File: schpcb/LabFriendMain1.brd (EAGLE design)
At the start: 100 x 100.1 mm, 654 parts, among them IC1 TPS62240DDC, IC10 TPS62240DDC, IC11 TPS73001DBVR, IC12 TPS73001DBVR, IC13 AK4621, IC14 TPS72301, IC15 LME49721, IC16 NE5532, IC17 OPA2134, IC18 LM8272, IC19 LMV358MM, IC2 25px80, IC20 ISL54405IRTZ, IC21 NE5532, IC22 74HC4052D, IC23 LME49721, IC24 74HC00D, IC25 INA331IDGK, IC26 MT41J128M8, IC27 74HCT132D, IC28 TPS72301, IC29 TPS73001DBVR, IC3 SI8462, IC30 LM8272, IC31 LMV358MM, IC32 ADS1118IDGSR, IC33 ADA4853-3RU, IC34 4052D, IC35 4052D, IC36 OPA2354, IC37 74HC595D, IC38 ADA4853-3RU, IC39 4052D, IC4 FT232H, IC40 4052D, IC41 OPA2354, IC42 74HC595D, IC43 LM321MF, IC44 74HC595D, IC5 ADC08200, IC6 ADC08200, IC7 TPS73001DBVR, IC8 93LC56SM, IC9 74LVC8T245, K1 G6K-2F-Y, K2 G6K-2F-Y, K3 G6K-2F-Y, K4 G6K-2F-Y, Q1 12MHz, Q2 FDN335N, Q3 FDN335N, T1 EFD15DCDCPM5P33EFD15, T10 BC850, T11 BC850, T12 BC856ASMD, T13 BC856ASMD, T14 BC850, T15 BC856ASMD, T16 BC850, T17 BC856ASMD, T2 BC850, T3 BC850, T4 BC850, T5 BC856ASMD, T6 BC856ASMD, T7 BC856ASMD, T8 BC850, T9 BC856ASMD, U2 6SLX9FTG256, X1 MINI-USB-32005-201, X2 31-5431-10RFX, X3 31-5431-10RFX

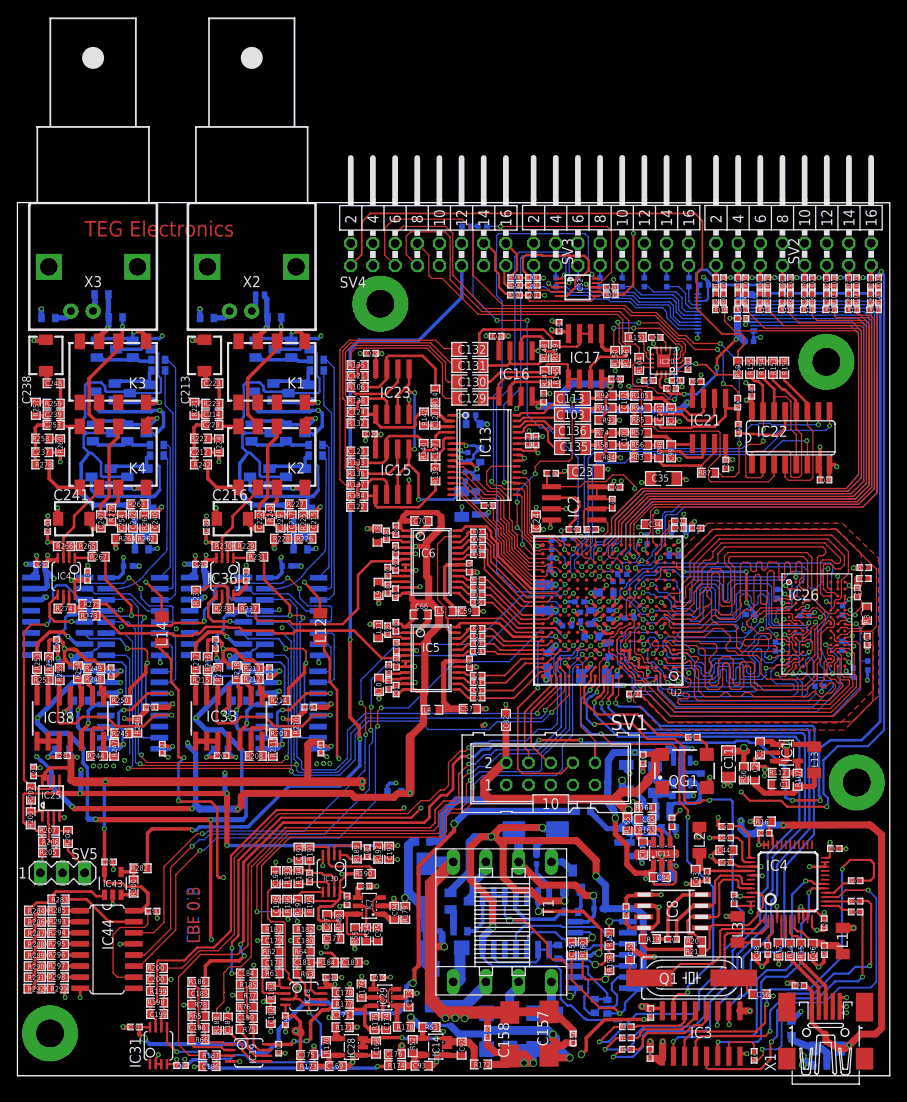
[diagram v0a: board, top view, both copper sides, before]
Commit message: Final oreder prototype
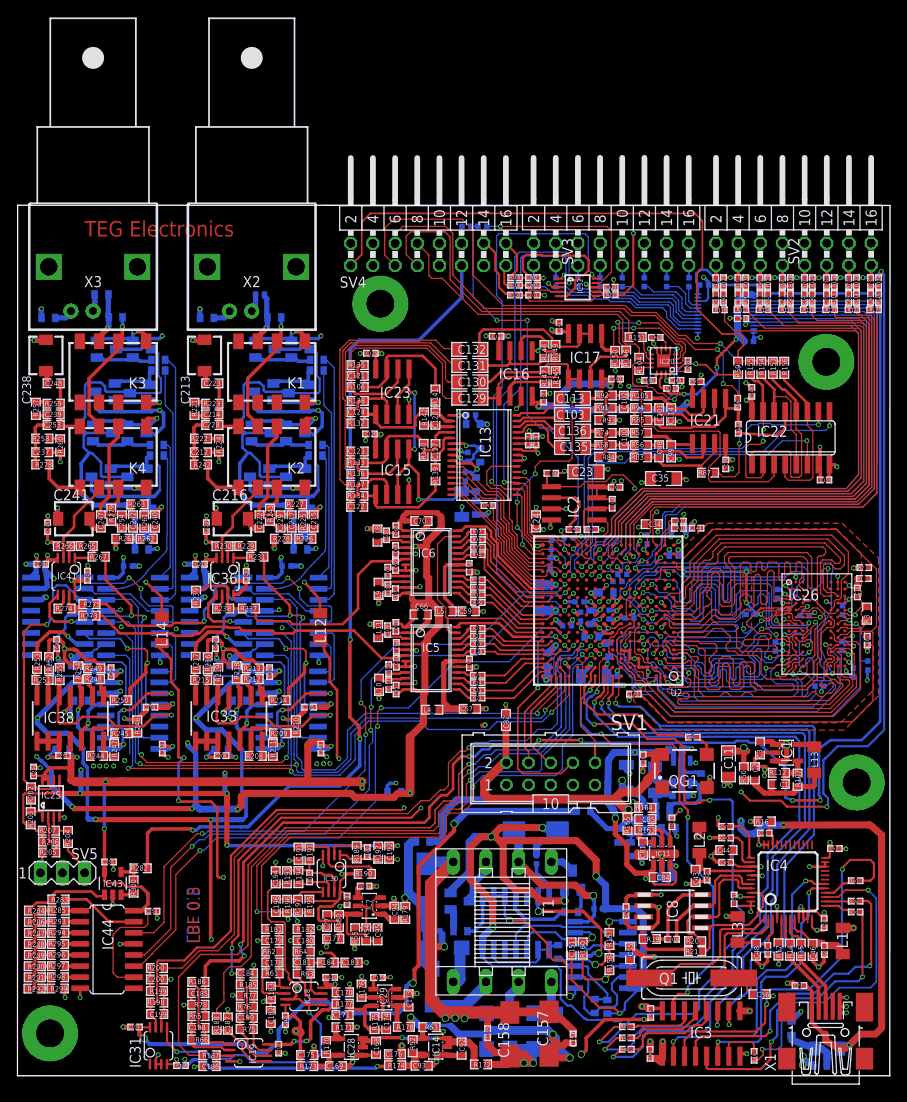
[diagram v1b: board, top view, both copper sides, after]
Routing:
- net VREFDDR: track 101.4 -> 100.4 mm
- added copper zone on layer 16, net VREFDDR
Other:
- board size 100 x 100.1 mm -> 100 x 99.8 mm
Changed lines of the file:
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@@
 <plain>
 <wire x1="60.2234" y1="0" x2="160.2032" y2="0" width="0" layer="20"/>
-<wire x1="160.2032" y1="0" x2="160.2032" y2="100.0508" width="0" layer="20"/>
-<wire x1="160.2032" y1="100.0508" x2="60.2234" y2="100.0762" width="0" layer="20"/>
-<wire x1="60.2234" y1="100.0762" x2="60.2234" y2="0" width="0" layer="20"/>
+<wire x1="160.2032" y1="0" x2="160.2282" y2="99.7508" width="0" layer="20"/>
+<wire x1="160.2282" y1="99.7508" x2="60.2484" y2="99.7762" width="0" layer="20"/>
+<wire x1="60.2484" y1="99.7762" x2="60.2234" y2="0" width="0" layer="20"/>
 <wire x1="119.0244" y1="58.0644" x2="119.0244" y2="57.8866" width="0" layer="47"/>
 <wire x1="83.6168" y1="22.1488" x2="83.4136" y2="22.1488" width="0" layer="47"/>
@@
 <vertex x="128.525" y="43.2"/>
 <vertex x="127.875" y="43.85"/>
-<vertex x="127.875" y="45.9875"/>
-<vertex x="128.2625" y="46.375"/>
-<vertex x="128.875" y="46.375"/>
-<vertex x="129.5125" y="47.0125"/>
-<vertex x="129.5125" y="49.8125"/>
-<vertex x="128.9375" y="49.975"/>
+<vertex x="127.9" y="45.7875"/>
+<vertex x="128.2375" y="46.175"/>
+<vertex x="129.175" y="46.175"/>
+<vertex x="129.175" y="46.525"/>
+<vertex x="129.0375" y="46.6625"/>
+<vertex x="128.5875" y="46.975"/>
+<vertex x="128.5375" y="49.775"/>
+<vertex x="128.375" y="49.9375"/>
 <vertex x="127.925" y="50"/>
 <vertex x="127.4875" y="50.3625"/>
@@
 <vertex x="129.725" y="55.0125"/>
 <vertex x="130.0125" y="54.575"/>
+<vertex x="129.95" y="51.2375"/>
+<vertex x="129.0125" y="50.225"/>
+<vertex x="129.0125" y="47.3125"/>
+<vertex x="129.975" y="46.35"/>
 <vertex x="129.975" y="45.7375"/>
 <vertex x="130.3625" y="45.35"/>
@@
 <via x="152.6865" y="18.7085" extent="1-16" drill="0.3048"/>
 <via x="151.003" y="23.9522" extent="1-16" drill="0.3048"/>
-<polygon width="0.254" layer="2" isolate="0.254">
+<polygon width="0.254" layer="2" isolate="0.15">
 <vertex x="137.2362" y="29.8704"/>
 <vertex x="136.9544" y="29.2612"/>
@@
 <via x="141.4526" y="18.288" extent="1-16" drill="0.3048"/>
 <via x="133.7726" y="19.3301" extent="1-16" drill="0.3048"/>
-<polygon width="0.2032" layer="3" isolate="0.254">
+<polygon width="0.2032" layer="3" isolate="0.15">
 <vertex x="152.2984" y="29.845"/>
 <vertex x="148.6662" y="29.8704"/>
@@
 <wire x1="156.45" y1="56.9999" x2="156.727" y2="57.0125" width="0.6096" layer="1"/>
 <contactref element="R50" pad="2"/>
-<polygon width="0.4064" layer="3" isolate="0.254">
-<vertex x="132.9625" y="42.6"/>
+<polygon width="0.4064" layer="3" isolate="0.15">
+<vertex x="132.4875" y="44.2625"/>
+<vertex x="131.8375" y="44.3"/>
+<vertex x="131.575" y="44.5625"/>
+<vertex x="129.425" y="44.5625"/>
+<vertex x="132.9375" y="41.05"/>
 <vertex x="132.9375" y="41"/>
 <vertex x="134.15" y="39.6125"/>
@@
 <vertex x="132.8375" y="49.8875"/>
 <vertex x="133.025" y="46.9375"/>
-<vertex x="132.95" y="43.625"/>
+<vertex x="133.05" y="44.675"/>
 </polygon>
 <wire x1="143.475" y1="35.4499" x2="143.475" y2="37.2125" width="0.6096" layer="1"/>
@@
 <wire x1="155.6625" y1="50.9375" x2="158.125" y2="50.9375" width="0.15" layer="1"/>
 <wire x1="158.125" y1="50.9375" x2="158.675" y2="51.4875" width="0.15" layer="1"/>
-<wire x1="148.65" y1="53.375" x2="148.3875" y2="53.375" width="0.15" layer="1"/>
-<wire x1="148.3875" y1="53.375" x2="148.3" y2="53.2875" width="0.15" layer="1"/>
-<wire x1="148.3" y1="53.2875" x2="145.7875" y2="53.2875" width="0.15" layer="1"/>
+<wire x1="148.65" y1="53.375" x2="148.5125" y2="53.375" width="0.15" layer="1"/>
+<wire x1="148.5125" y1="53.375" x2="148.425" y2="53.2875" width="0.15" layer="1"/>
+<wire x1="148.425" y1="53.2875" x2="145.7875" y2="53.2875" width="0.15" layer="1"/>
 <wire x1="145.7875" y1="53.2875" x2="145.425" y2="52.9375" width="0.15" layer="1"/>
 <wire x1="145.425" y1="52.9375" x2="145.2875" y2="52.9375" width="0.15" layer="1"/>
-<wire x1="145.2875" y1="52.9375" x2="144.725" y2="52.175" width="0.15" layer="1"/>
-<via x="144.725" y="52.175" extent="1-16" drill="0.3"/>
-<wire x1="144.725" y1="52.175" x2="144.725" y2="53.125" width="0.15" layer="16"/>
-<wire x1="144.725" y1="53.125" x2="143.775" y2="54.225" width="0.3048" layer="16"/>
+<wire x1="145.2875" y1="52.9375" x2="145.4375" y2="52.9" width="0.15" layer="1"/>
+<via x="145.4375" y="52.9" extent="1-16" drill="0.3"/>
+<wire x1="145.4375" y1="52.9" x2="144.725" y2="53.125" width="0.15" layer="16"/>
+<wire x1="144.725" y1="53.125" x2="144.725" y2="53.175" width="0.3048" layer="16"/>
+<wire x1="144.725" y1="53.175" x2="143.8375" y2="54.0625" width="0.3048" layer="16"/>
+<wire x1="143.8375" y1="54.0625" x2="143.775" y2="54.225" width="0.3048" layer="16"/>
 <via x="143.775" y="54.225" extent="1-16" drill="0.3"/>
 <wire x1="143.775" y1="54.225" x2="143.775" y2="56.925" width="0.3048" layer="1"/>
@@
 <vertex x="131.675" y="45.0125"/>
 </polygon>
-<wire x1="144.7605" y1="52.875" x2="144.7605" y2="52.2105" width="0.4064" layer="16"/>
-<wire x1="144.7605" y1="52.2105" x2="144.725" y2="52.175" width="0.4064" layer="16"/>
+<wire x1="144.7605" y1="52.875" x2="144.923" y2="52.898" width="0.4064" layer="16"/>
+<wire x1="144.923" y1="52.898" x2="145.4375" y2="52.9" width="0.4064" layer="16"/>
 <contactref element="R2" pad="2"/>
 <contactref element="R1" pad="1"/>
+<polygon width="0.15" layer="1" isolate="0.15">
+<vertex x="145.3125" y="52.7"/>
+<vertex x="145.6125" y="52.7"/>
+<vertex x="145.9" y="52.4125"/>
+<vertex x="146.3625" y="52.4125"/>
+<vertex x="146.9875" y="53.0375"/>
+<vertex x="148.5875" y="53.0375"/>
+<vertex x="148.9125" y="53.3625"/>
+<vertex x="148.9125" y="53.4625"/>
+<vertex x="148.6875" y="53.6875"/>
+<vertex x="148.225" y="53.6875"/>
+<vertex x="148.075" y="53.5375"/>
+<vertex x="145.425" y="53.5375"/>
+<vertex x="145.125" y="53.2375"/>
+<vertex x="145.125" y="52.8875"/>
+</polygon>
+<polygon width="0.15" layer="1" isolate="0.15">
+<vertex x="143.7875" y="54.2"/>
+<vertex x="144.175" y="54.2"/>
+<vertex x="144.375" y="54.4"/>
+<vertex x="144.375" y="57.5125"/>
+<vertex x="143.9125" y="57.975"/>
+<vertex x="143.55" y="57.975"/>
+<vertex x="143.3625" y="57.7875"/>
+<vertex x="143.3625" y="54.575"/>
+<vertex x="143.7375" y="54.2"/>
+</polygon>
+<polygon width="0.15" layer="16" isolate="0.15">
+<vertex x="136.725" y="57.25"/>
+<vertex x="143.6625" y="57.25"/>
+<vertex x="144.075" y="57.6625"/>
+<vertex x="144.075" y="58.05"/>
+<vertex x="143.95" y="58.175"/>
+<vertex x="136.775" y="58.175"/>
+<vertex x="136.5125" y="57.9125"/>
+<vertex x="136.5125" y="57.5"/>
+<vertex x="136.75" y="57.2625"/>
+</polygon>
 </signal>
 <signal name="CASN">
@@
 <wire x1="132.15" y1="52.3375" x2="132.6625" y2="51.9" width="0.15" layer="16"/>
 <wire x1="150.25" y1="51.775" x2="150.25" y2="51.7875" width="0.15" layer="1"/>
-<via x="145.525" y="52.1625" extent="1-16" drill="0.3"/>
-<wire x1="145.525" y1="52.1625" x2="145.4625" y2="52.1" width="0.15" layer="16"/>
-<wire x1="145.525" y1="52.1625" x2="145.525" y2="52.3" width="0.15" layer="1"/>
-<wire x1="145.525" y1="52.3" x2="146.2" y2="52.975" width="0.15" layer="1"/>
-<wire x1="146.2" y1="52.975" x2="148.8875" y2="52.975" width="0.15" layer="1"/>
+<via x="145.5" y="52.1375" extent="1-16" drill="0.3"/>
+<wire x1="145.5" y1="52.1375" x2="145.4625" y2="52.1" width="0.15" layer="16"/>
 <wire x1="148.8875" y1="52.975" x2="149.05" y2="52.8125" width="0.15" layer="1"/>
 <wire x1="149.05" y1="52.8125" x2="149.05" y2="52.4" width="0.15" layer="1"/>
@@
 <wire x1="135.9125" y1="50.4375" x2="136.15" y2="50.2" width="0.15" layer="16"/>
 <wire x1="136.15" y1="50.2" x2="143.5625" y2="50.2" width="0.15" layer="16"/>
-<wire x1="143.5625" y1="50.2" x2="145.525" y2="52.1625" width="0.15" layer="16"/>
+<wire x1="143.5625" y1="50.2" x2="145.5" y2="52.1375" width="0.15" layer="16"/>
+<wire x1="145.5" y1="52.1375" x2="146.3875" y2="52.1375" width="0.15" layer="1"/>
+<wire x1="146.3875" y1="52.1375" x2="147.05" y2="52.8" width="0.15" layer="1"/>
+<wire x1="147.05" y1="52.8" x2="147.6875" y2="52.8" width="0.15" layer="1"/>
+<wire x1="147.6875" y1="52.8" x2="147.75" y2="52.8625" width="0.15" layer="1"/>
+<wire x1="147.75" y1="52.8625" x2="148.1875" y2="52.8625" width="0.15" layer="1"/>
+<wire x1="148.1875" y1="52.8625" x2="148.3" y2="52.975" width="0.15" layer="1"/>
+<wire x1="148.3" y1="52.975" x2="148.8875" y2="52.975" width="0.15" layer="1"/>
 </signal>
 <signal name="RASN">

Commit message: many improovments and bugfixes and added features
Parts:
- R261: value 51k -> 130k
- R262: value 39k -> 47k
- R263: value 910k -> 820k
- R264: value 1k -> 3k
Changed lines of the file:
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@@
 <?xml version="1.0" encoding="utf-8"?>
 <!DOCTYPE eagle SYSTEM "eagle.dtd">
-<eagle version="7.3.0">
+<eagle version="7.7.0">
 <drawing>
 <settings>
@@
 <attribute name="NAME" x="63.3316" y="75.4962" size="0.6096" layer="25" ratio="10"/>
 </element>
-<element name="R261" library="passive" package="0603" value="51k" x="74.7616" y="63.5328" smashed="yes" rot="R90">
+<element name="R261" library="passive" package="0603" value="130k" x="74.7616" y="63.5328" smashed="yes" rot="R90">
 <attribute name="VALUE" x="72.8566" y="62.3898" size="0.8128" layer="27" ratio="10" rot="R90"/>
 <attribute name="NAME" x="75.0918" y="62.4914" size="0.6096" layer="25" ratio="10" rot="R90"/>
@@
 <attribute name="NAME" x="75.676" y="64.5996" size="0.6096" layer="25" ratio="10" rot="R270"/>
 </element>
-<element name="R262" library="passive" package="0603" value="39k" x="75.041" y="61.5516" smashed="yes">
+<element name="R262" library="passive" package="0603" value="47k" x="75.041" y="61.5516" smashed="yes">
 <attribute name="VALUE" x="73.898" y="63.4566" size="0.8128" layer="27" ratio="10"/>
 <attribute name="NAME" x="73.9742" y="61.2468" size="0.6096" layer="25" ratio="10"/>
@@
 <attribute name="VALUE" x="60.3344" y="66.3776" size="1.27" layer="27" rot="R270"/>
 </element>
-<element name="R263" library="passive" package="0603" value="910k" x="73.977790625" y="65.49746875" smashed="yes" rot="R180">
+<element name="R263" library="passive" package="0603" value="820k" x="73.977790625" y="65.49746875" smashed="yes" rot="R180">
 <attribute name="VALUE" x="75.12079375" y="63.59246875" size="0.8128" layer="27" ratio="10" rot="R180"/>
 <attribute name="NAME" x="72.89865625" y="65.204996875" size="0.6096" layer="25" ratio="10"/>
 </element>
-<element name="R264" library="passive" package="0603" value="1k" x="72.247" y="61.5516" smashed="yes">
+<element name="R264" library="passive" package="0603" value="3k" x="72.247" y="61.5516" smashed="yes">
 <attribute name="VALUE" x="71.104" y="63.4566" size="0.8128" layer="27" ratio="10"/>
 <attribute name="NAME" x="71.7898" y="61.2722" size="0.6096" layer="25" ratio="10"/>
@@
 <contactref element="SV1" pad="3"/>
 <contactref element="R9" pad="2"/>
-<contactref element="IC2" pad="4"/>
 <contactref element="C33" pad="2"/>
 <contactref element="C34" pad="2"/>
@@
 <contactref element="C185" pad="2"/>
 <contactref element="C187" pad="2"/>
-<contactref element="C187" pad="2"/>
-<contactref element="C186" pad="2"/>
 <contactref element="C186" pad="2"/>
 <contactref element="IC30" pad="4"/>
@@
 <wire x1="94.6967" y1="76.2582" x2="95.1539" y2="75.9534" width="0.4064" layer="16"/>
 <wire x1="93.7823" y1="66.3776" x2="94.1125" y2="66.403" width="0.4064" layer="16"/>
-<contactref element="IC37" pad="8"/>
 <contactref element="C221" pad="1"/>
 <wire x1="83.1905" y1="38.3522" x2="81.9205" y2="38.3522" width="0.6096" layer="1"/>
@@
 <wire x1="76.5142" y1="76.2582" x2="76.9714" y2="75.9534" width="0.4064" layer="16"/>
 <wire x1="75.5998" y1="66.3776" x2="75.93" y2="66.403" width="0.4064" layer="16"/>
-<contactref element="IC42" pad="8"/>
 <contactref element="C246" pad="1"/>
 <wire x1="65.008" y1="38.3522" x2="63.738" y2="38.3522" width="0.6096" layer="1"/>
@@
 <contactref element="C51" pad="1"/>
 <contactref element="IC4" pad="46"/>
-<contactref element="IC4" pad="24"/>
-<contactref element="IC4" pad="12"/>
 <contactref element="R16" pad="2"/>
 <contactref element="R19" pad="2"/>
